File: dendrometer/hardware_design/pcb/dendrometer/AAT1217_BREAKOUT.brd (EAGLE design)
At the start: 14.3 x 13.2 mm, 7 parts

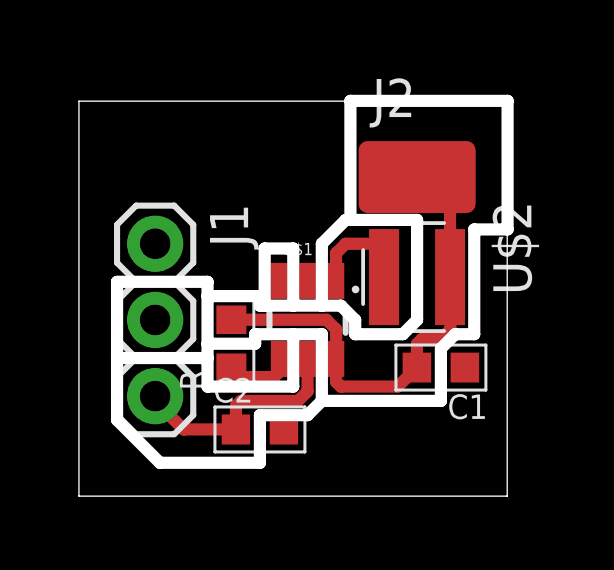
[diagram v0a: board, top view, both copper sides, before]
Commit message: minor code updates...
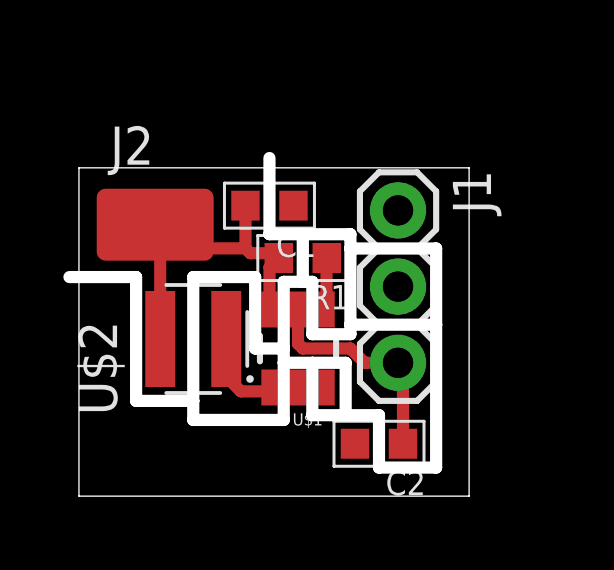
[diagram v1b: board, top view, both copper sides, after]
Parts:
- moved J2 8.87 mm to (2.54, 9.05)
- moved J1 8.17 mm to (10.6, 9.53)
- moved C1 7.86 mm to (6.35, 9.68)
- moved U$2 7.74 mm to (3.81, 5.24), turned to 90 degrees
- moved C2 4.00 mm to (10.0, 1.75), turned to 180 degrees
- moved R1 3.72 mm to (7.46, 7.94), turned to 180 degrees
- moved U$1 1.00 mm to (7.30, 4.92), turned to 180 degrees
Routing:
- net N$2: track 16.0 -> 11.4 mm
- net N$4: track 3.76 -> 2.96 mm
- net N$1: track 2.23 -> 1.72 mm
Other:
- board size 14.3 x 13.2 mm -> 13.3 x 11.3 mm
